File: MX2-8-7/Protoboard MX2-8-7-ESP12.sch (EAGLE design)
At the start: 144 parts, among them J1 DCJ0202

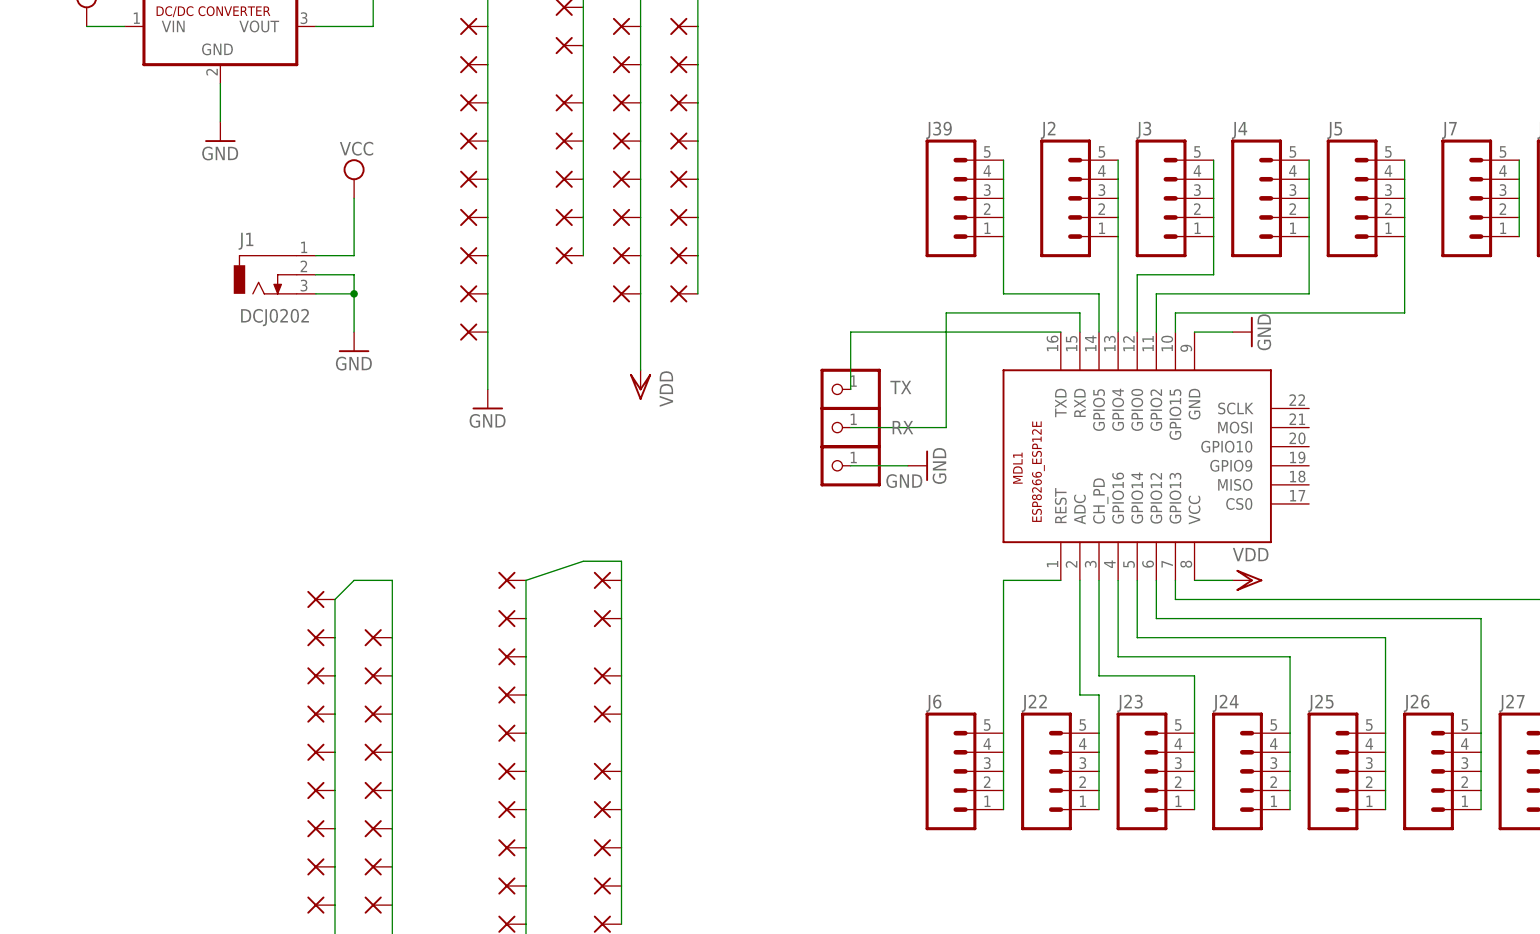
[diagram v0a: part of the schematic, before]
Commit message: Update esp component and usb
test
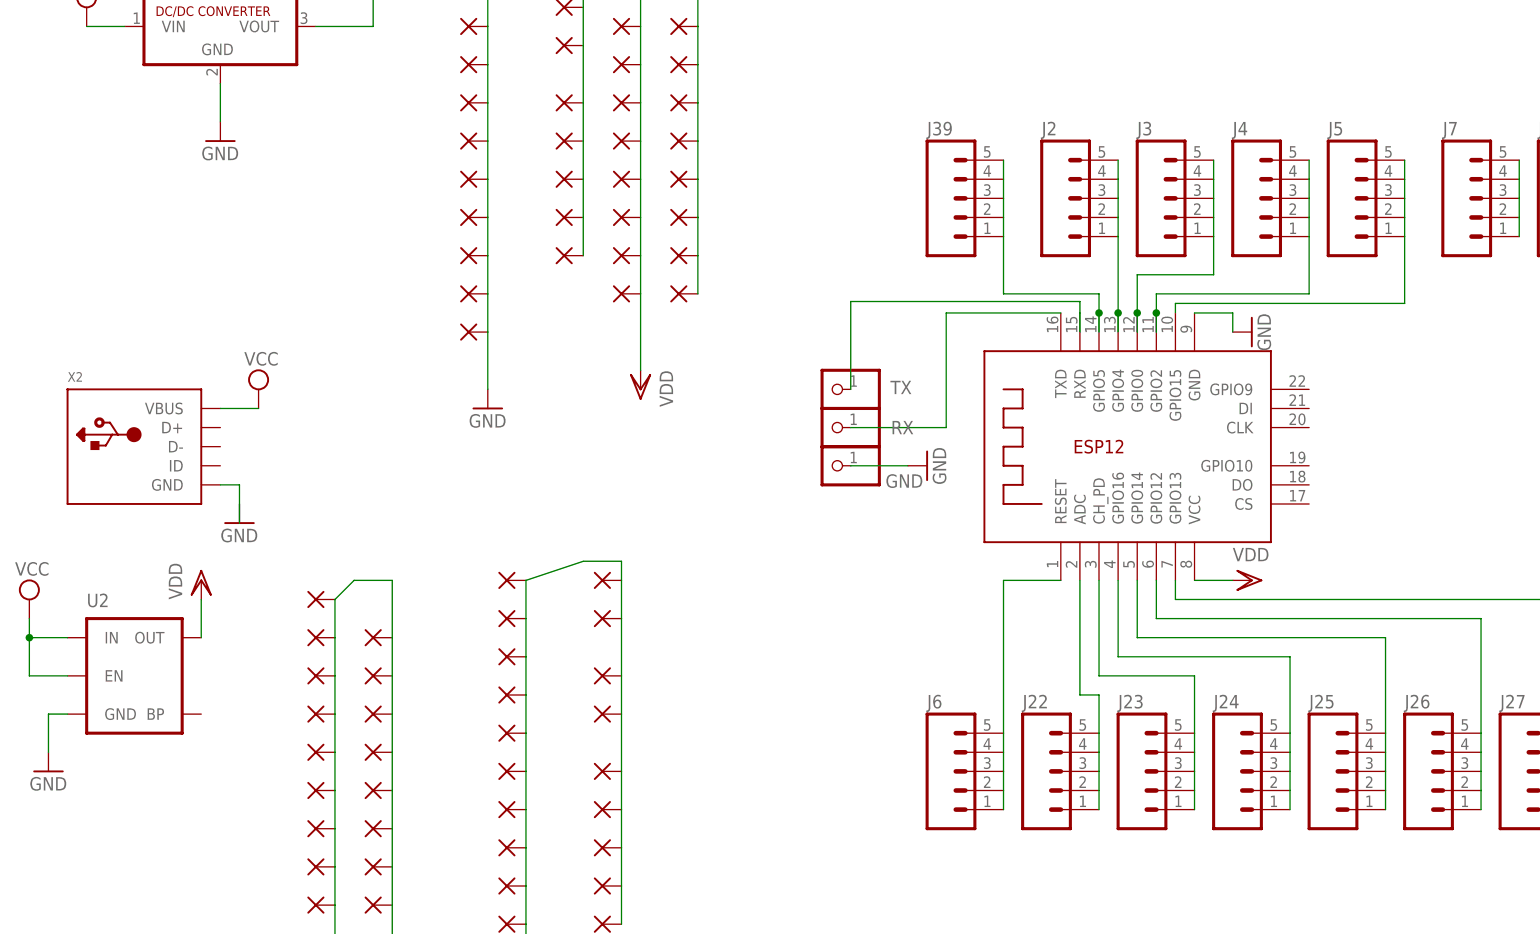
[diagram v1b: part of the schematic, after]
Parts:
- removed J1: DCJ0202, con-jack:DCJ0202
- removed MDL1: (no value), ESP8266-ESP12E:ESP8266-12EESP8266-ESP12E
- added U2: (no value), SparkFun-PowerIC:MIC52053.3V
- added X1: ESP-12E, microbuilder:ESP-12E
- added X2: (no value), microbuilder:USB_MICRO_20329_V2
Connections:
- new net N$45: TX.1, X1.RXD
- net GND: now also U2.GND, X1.GND; no longer J1.2, J1.3, MDL1.GND
- net N$1: now also X1.GPIO5; no longer MDL1.GPIO5
- net N$22: now also X1.RESET; no longer MDL1.REST
- net N$23: now also X1.ADC; no longer MDL1.ADC
- net N$24: now also X1.CH_PD; no longer MDL1.CH_PD
- net N$25: now also X1.GPIO16; no longer MDL1.GPIO16
- net N$26: now also X1.GPIO14; no longer MDL1.GPIO14
- net N$27: now also X1.GPIO12; no longer MDL1.GPIO12
- net N$28: now also X1.GPIO13; no longer MDL1.GPIO13
- net N$3: now also X1.GPIO4; no longer MDL1.GPIO4
- net N$4: now also X1.GPIO0; no longer MDL1.GPIO0
- net N$46: now also X1.TXD; no longer MDL1.RXD
- net N$47: now also X2.GND; no longer MDL1.TXD, TX.1
- net N$5: now also X1.GPIO2; no longer MDL1.GPIO2
- net N$6: now also X1.GPIO15; no longer MDL1.GPIO15
- net VCC: now also U2.EN, U2.IN, X2.VBUS; no longer J1.1
- net VDD: now also U2.OUT, X1.VCC; no longer MDL1.VCC
